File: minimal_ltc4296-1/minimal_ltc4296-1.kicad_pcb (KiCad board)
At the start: 4 copper layers, 15.2 x 15.2 mm, 2 parts, among them U1 LTC4296AUK-1-PBF

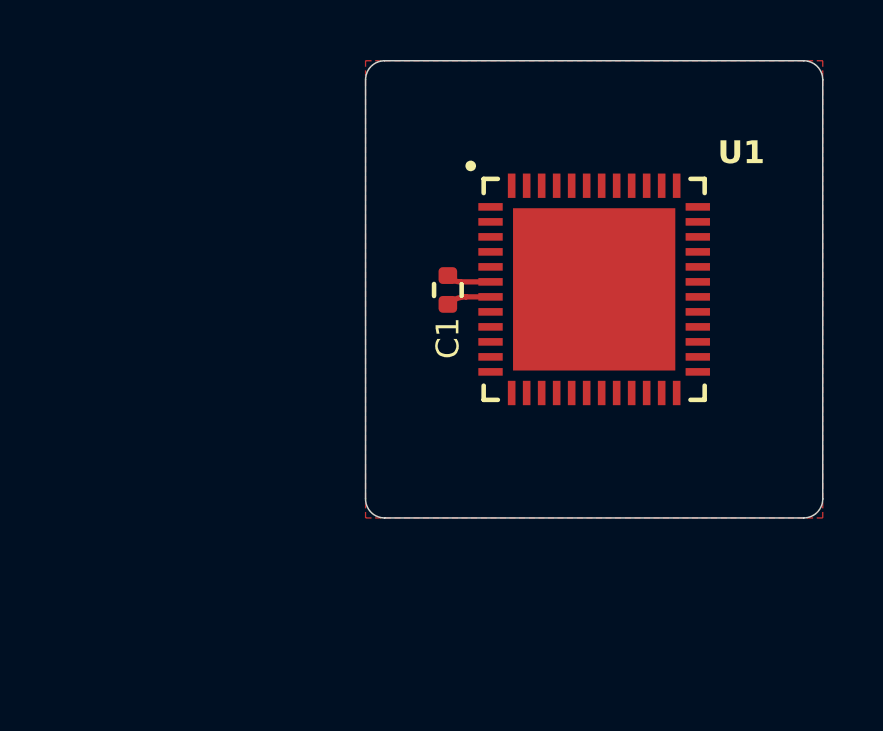
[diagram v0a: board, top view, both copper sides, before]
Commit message: Update KiCAD files and submodule
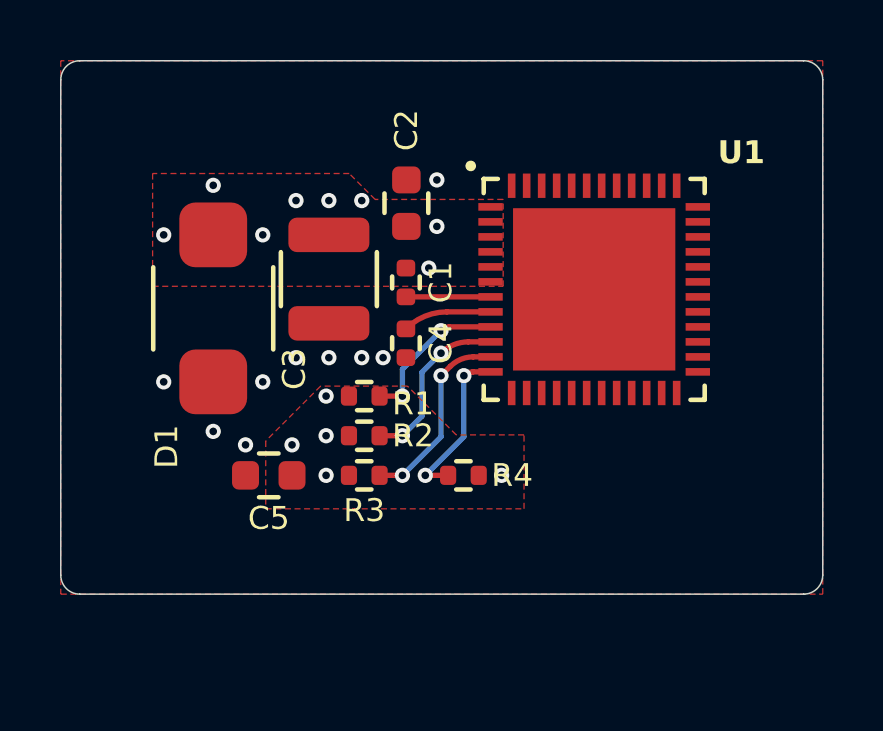
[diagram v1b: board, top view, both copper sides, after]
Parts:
- added C2: 100 nF, capacitor_footprints:C_0603_1608Metric, F.Cu at (143.4, 99.5)
- added C3: 10 µF, capacitor_footprints:C_1210_250_3225Metric, F.Cu at (140.9, 102.0)
- added C4: 470 nF, capacitor_footprints:C_0402_1005Metric, F.Cu at (143.4, 104.2)
- added C5: 100 nF, capacitor_footprints:C_0603_1608Metric, F.Cu at (138.9, 108.6)
- added D1: 58 V, diode_footprints:DO-214AA, F.Cu at (137.0, 103.0)
- added R1: 10 kΩ, resistor_footprints:R_0402_1005Metric, F.Cu at (142.0, 105.9)
- added R2: 4.99 kΩ, resistor_footprints:R_0402_1005Metric, F.Cu at (142.0, 107.2)
- added R3: 10 kΩ, resistor_footprints:R_0402_1005Metric, F.Cu at (142.0, 108.6)
- added R4: 10 kΩ, resistor_footprints:R_0402_1005Metric, F.Cu at (145.4, 108.6)
- moved C1 1.42 mm to (143.4, 102.1)
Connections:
- U1 pad 10: unconnected-(U1-SDO-Pad10) -> /SDO
- U1 pad 11: unconnected-(U1-SCK-Pad11) -> /SCK
- U1 pad 12: unconnected-(U1-~{CS}-Pad12) -> /~{CS}
- U1 pad 8: unconnected-(U1-INT-Pad8) -> /INT
- U1 pad 9: unconnected-(U1-SDI-Pad9) -> /SDI
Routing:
- net /SCK: track 0.00 -> 6.48 mm, vias 0 -> 2
- net /SDO: track 0.00 -> 5.79 mm, vias 0 -> 2
- net /~{CS}: track 0.00 -> 5.54 mm, vias 0 -> 2
- net /SDI: track 0.00 -> 5.16 mm, vias 0 -> 2
- net /INT: track 0.00 -> 2.96 mm
- net /IN: track 1.49 -> 0.00 mm, vias 0 -> 8
- net /CPO: track 1.49 -> 2.82 mm
- net GND: vias 0 -> 9
- net /3V3: vias 0 -> 5
- added copper zone on F.Cu, net /3V3
- added copper zone on F.Cu, net /IN
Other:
- board size 15.2 x 15.2 mm -> 25.4 x 17.8 mm

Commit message: Update KiCAD files and submodule
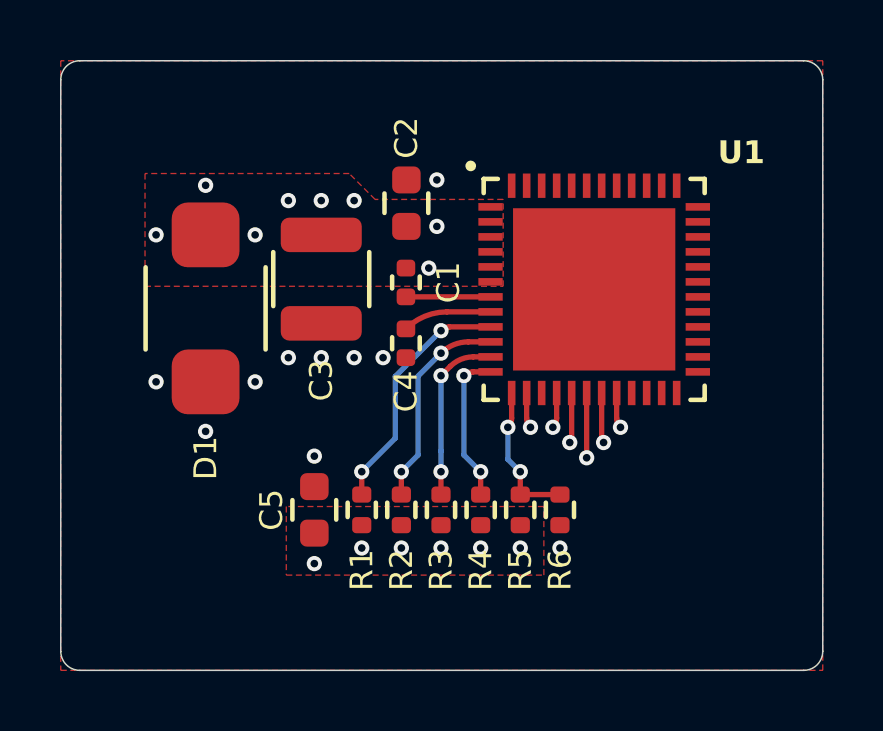
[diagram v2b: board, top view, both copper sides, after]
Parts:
- added R5: 100 kΩ, resistor_footprints:R_0402_1005Metric, F.Cu at (147.2, 109.7)
- added R6: 100 kΩ, resistor_footprints:R_0402_1005Metric, F.Cu at (148.6, 109.7)
- moved R1 3.79 mm to (142.0, 109.7), turned to 90 degrees
- moved R3 2.80 mm to (144.6, 109.7), turned to 90 degrees
- moved R2 2.76 mm to (143.3, 109.7), turned to 90 degrees
- moved C5 1.91 mm to (140.4, 109.7), turned to 90 degrees
- moved R4 1.29 mm to (145.9, 109.7), turned to 90 degrees
- moved D1 0.25 mm to (136.8, 103.0)
- moved C3 0.25 mm to (140.6, 102.0)
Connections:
- U1 pad 13: unconnected-(U1-AUTO-Pad13) -> /AUTO
- U1 pad 14: unconnected-(U1-WAKEUP-Pad14) -> /WAKEUP
- U1 pad 16: unconnected-(U1-SW0-Pad16) -> /SW0
- U1 pad 17: unconnected-(U1-SW1-Pad17) -> /SW1
- U1 pad 18: unconnected-(U1-SW2-Pad18) -> /SW2
- U1 pad 19: unconnected-(U1-SW3-Pad19) -> /SW3
- U1 pad 20: unconnected-(U1-SW4-Pad20) -> /SW4
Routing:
- net /AUTO: track 0.00 -> 4.91 mm, vias 0 -> 2
- net /SDI: track 5.16 -> 8.24 mm
- net /SW2: track 0.00 -> 2.16 mm, vias 0 -> 1
- net /SW3: track 0.00 -> 1.67 mm, vias 0 -> 1
- net /SW1: track 0.00 -> 1.67 mm, vias 0 -> 1
- net /SDO: track 5.79 -> 7.01 mm
- net /SW0: track 0.00 -> 1.17 mm, vias 0 -> 1
- net /WAKEUP: track 0.00 -> 1.17 mm, vias 0 -> 1
- net /SW4: track 0.00 -> 1.17 mm, vias 0 -> 1
- net /SCK: track 6.48 -> 5.82 mm
- net GND: vias 9 -> 10
- net /3V3: vias 5 -> 6
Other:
- board size 25.4 x 17.8 mm -> 25.4 x 20.3 mm
